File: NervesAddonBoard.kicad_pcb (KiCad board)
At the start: 2 copper layers, 65 x 30 mm, 10 parts, among them IC1 ATECC608A-SSHDA-B, J1 Conn_02x20_Odd_Even, J2 Grove_4pin_connector, J3 Grove_4pin_connector, J4 Grove_4pin_connector

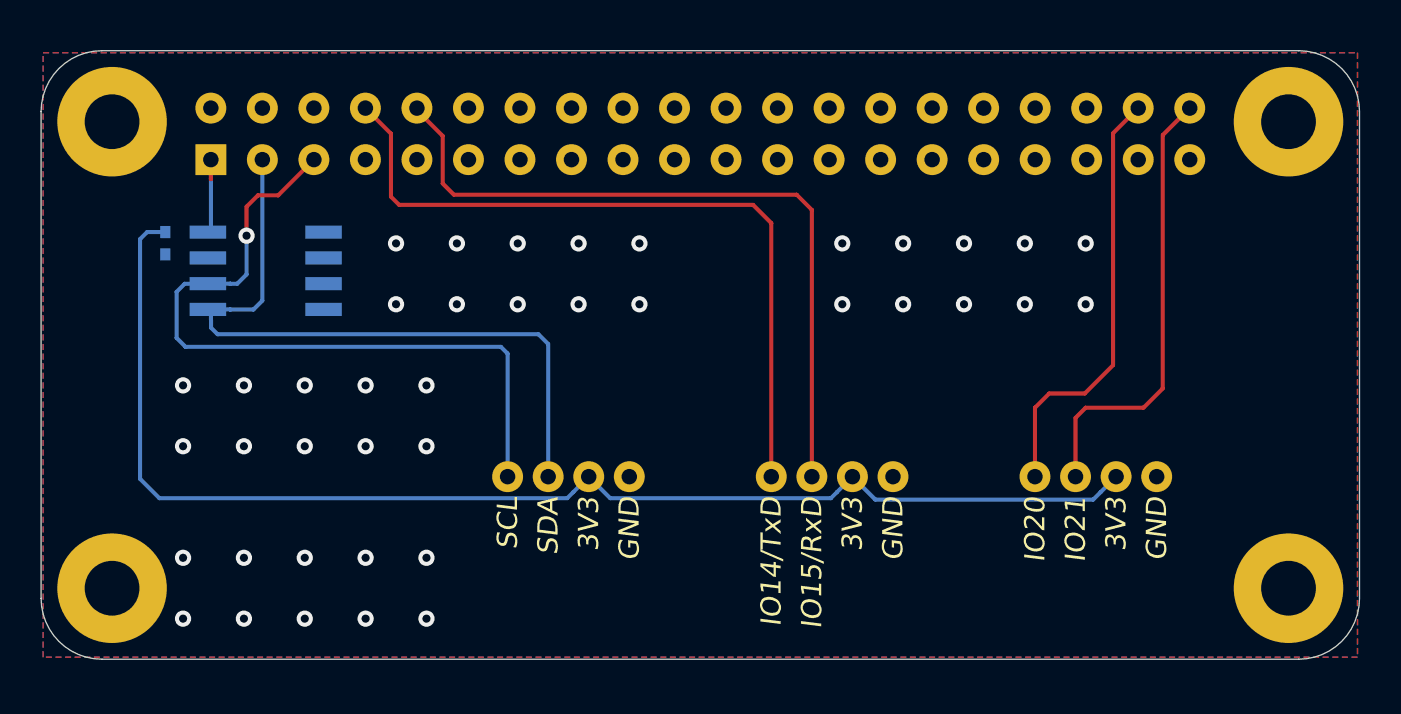
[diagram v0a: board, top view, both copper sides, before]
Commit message: update
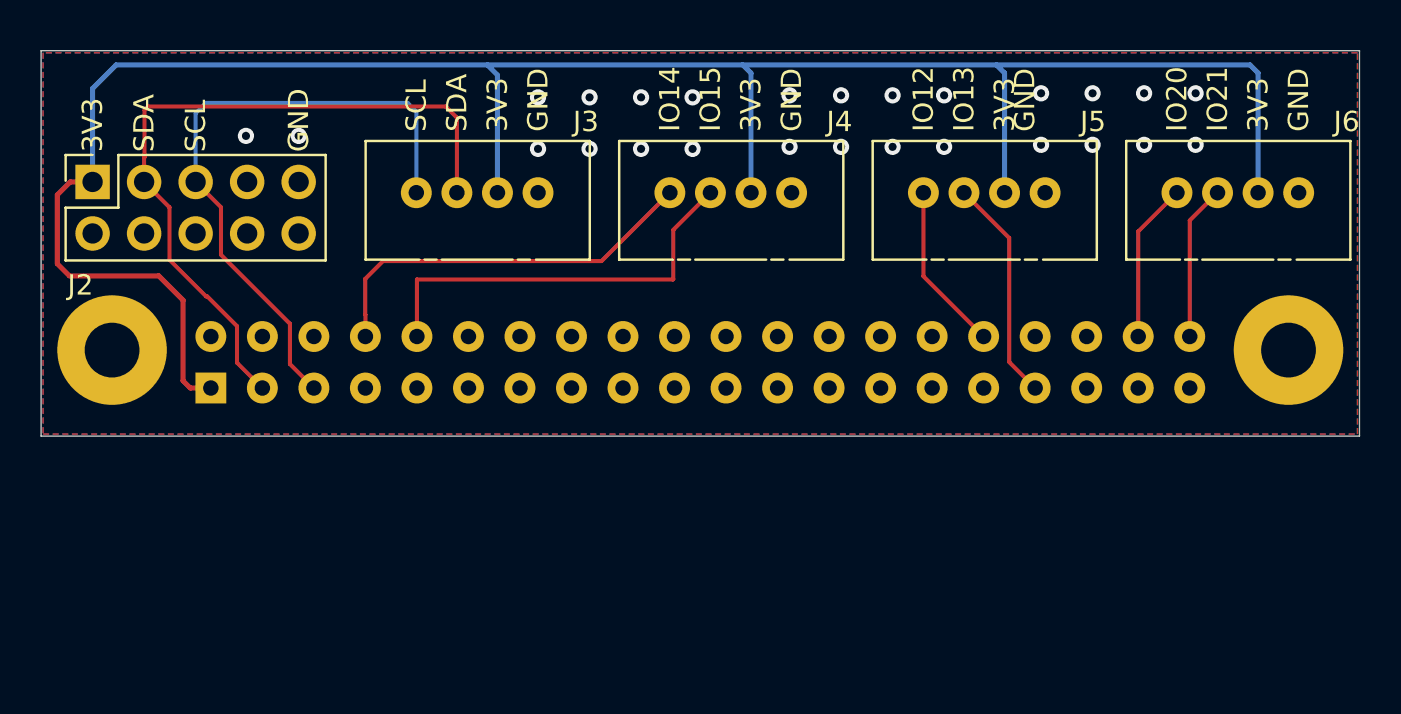
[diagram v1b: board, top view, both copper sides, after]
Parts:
- removed C1: C, NervesAddonBoard.foot:C_0402
- removed IC1: ATECC608A-SSHDA-B, NervesAddonBoard.foot:SOIC127P600X175-8N
- removed the REF** at (81.5, 23.5)
- removed the REF** at (81.5, 46.5)
- removed the REF** at (23.5, 46.5)
- removed the REF** at (23.5, 23.5)
- added J5: Grove_4pin_connector, NervesAddonBoard.foot:Grove_1x04, F.Cu at (63.5, 27.0)
- added J6: Grove_4pin_connector, NervesAddonBoard.foot:Grove_1x04, F.Cu at (76.0, 27.0)
- added REF**: MountingHole_2.7mm_M2.5_Pad, Mounting_Holes:MountingHole_2.7mm_M2.5_Pad, F.Cu at (81.5, 34.8)
- added REF**: MountingHole_2.7mm_M2.5_Pad, Mounting_Holes:MountingHole_2.7mm_M2.5_Pad, F.Cu at (23.5, 34.8)
- J2: value Grove_4pin_connector -> Conn_02x05_Odd_Even; footprint NervesAddonBoard.foot:Grove_1x04_90 -> NervesAddonBoard.foot:Socket_Strip_Straight_2x05_Pitch2.54mm; moved to F.Cu
- J3, J4: footprint NervesAddonBoard.foot:Grove_1x04_90 -> NervesAddonBoard.foot:Grove_1x04; moved to F.Cu
- moved J2 25.1 mm to (22.5, 26.5), turned to 90 degrees
- moved J4 22.8 mm to (51.0, 27.0), turned to 90 degrees
- moved J3 22.4 mm to (38.5, 27.0), turned to 90 degrees
- moved J1 11.3 mm to (28.4, 36.6)
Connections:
- J1 pad 32: Net-(J1-Pad32) -> /IO12_PWM0
- J1 pad 33: Net-(J1-Pad33) -> /IO13_PWM1
- J2 pad 1: /SCL -> +3V3
- J2 pad 2: /SDA -> Net-(J2-Pad2)
- J2 pad 3: +3V3 -> /SDA
- J2 pad 4: GND -> Net-(J2-Pad4)
- J3 pad 1: /IO14_TxD -> /SCL
- J3 pad 2: /IO15_RxD -> /SDA
- J4 pad 1: /IO20 -> /IO14_TxD
- J4 pad 2: /IO21 -> /IO15_RxD
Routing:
- net +3V3: track 68.5 -> 106.9 mm
- net /IO14_TxD: track 36.7 -> 19.6 mm
- net /IO15_RxD: track 36.2 -> 20.5 mm
- net /IO21: track 22.2 -> 7.66 mm
- net /IO20: track 21.3 -> 7.88 mm
- net /IO13_PWM1: track 0.00 -> 11.1 mm
- net /IO12_PWM0: track 0.00 -> 8.32 mm
- net /SCL: track 36.4 -> 31.2 mm, vias 1 -> 0
- net /SDA: track 34.1 -> 35.6 mm
- net GND: vias 40 -> 26
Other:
- board size 65 x 30 mm -> 65 x 19 mm
- board text added: "IO12"
- board text added: "IO13"
- board text added: "IO14"
- board text added: "IO15"
- board text removed: "IO14/TxD"
- board text removed: "IO15/RxD"
